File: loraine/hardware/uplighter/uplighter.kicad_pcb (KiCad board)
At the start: 2 copper layers, 50 x 50 mm, 13 parts, among them K1 CONN_3, K2 CONN_3, K3 CONN_3, U1 TL4242, U2 TL4242, U3 TL4242

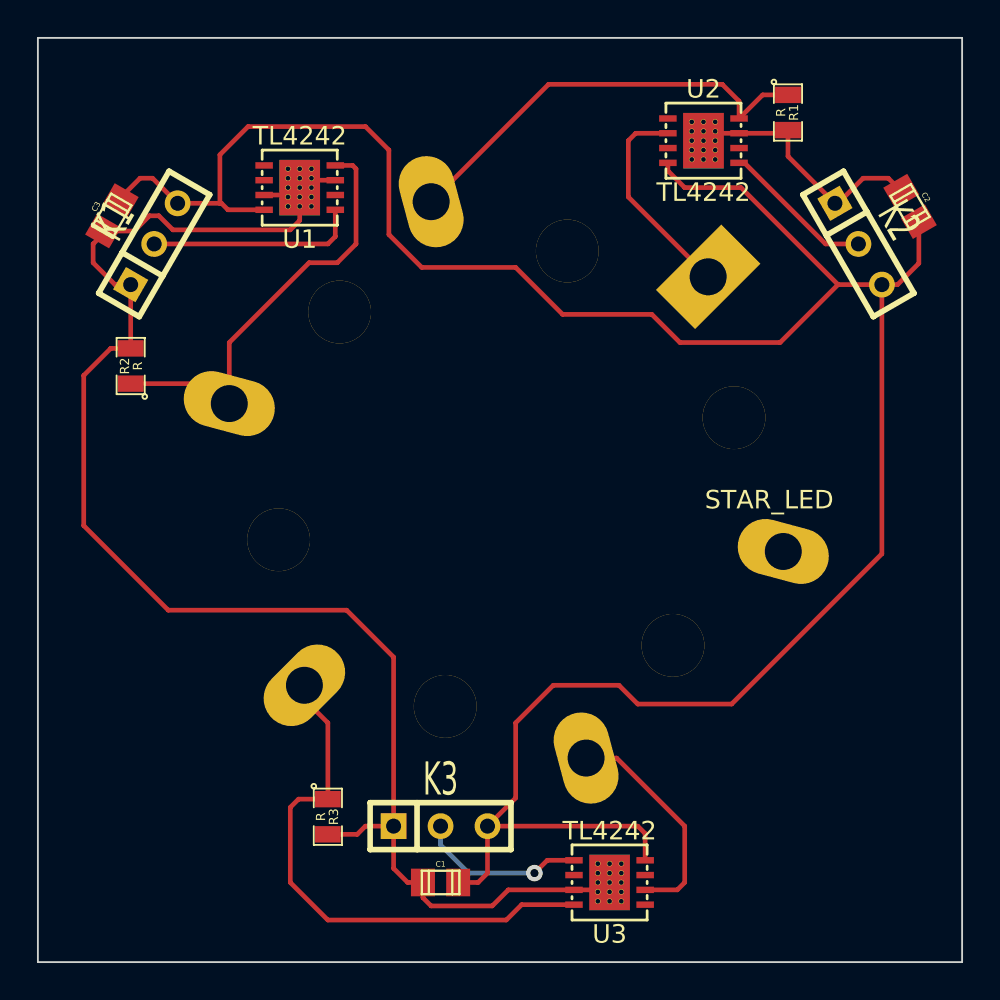
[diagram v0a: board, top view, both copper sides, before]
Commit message: Finished both PCBs apart from logos and checking
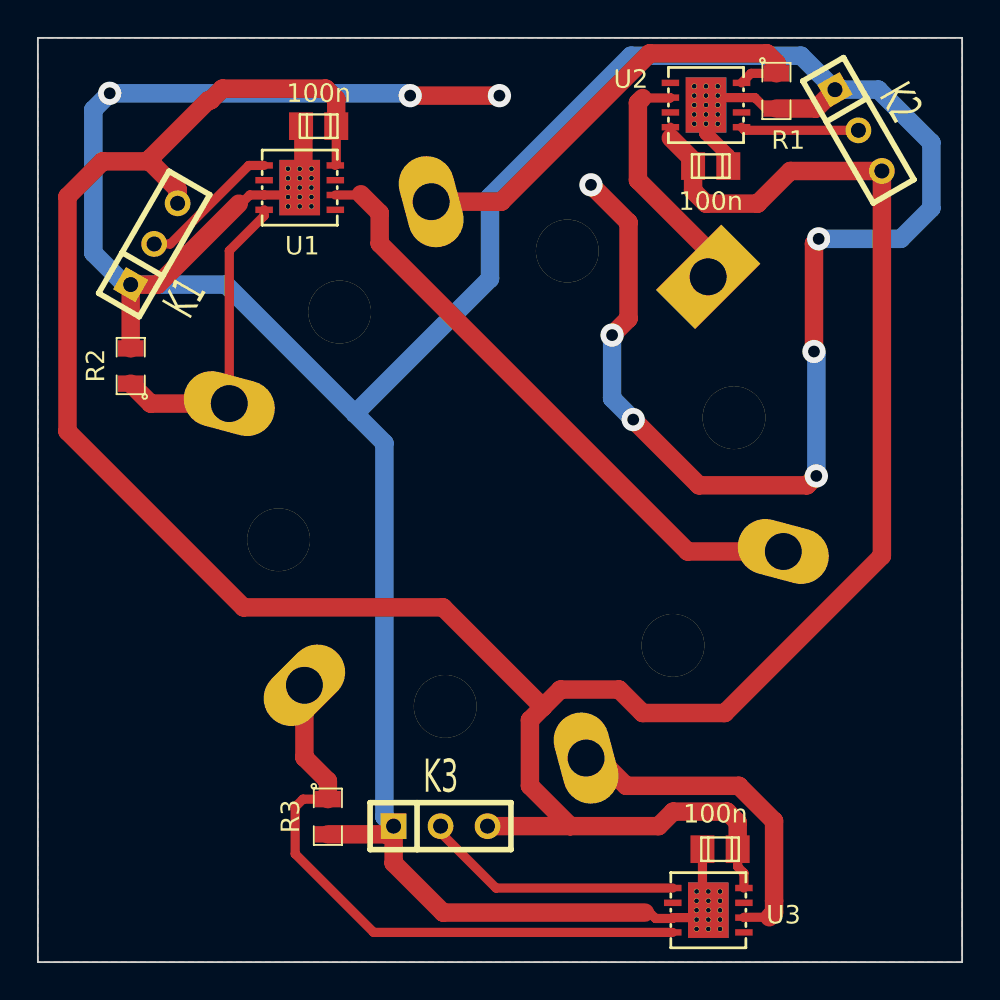
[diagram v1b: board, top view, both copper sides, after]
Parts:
- C1, C2, C3: value C -> 100n
- moved C1 15.2 mm to (136.9, 143.9)
- moved C3 12.2 mm to (115.2, 104.8), turned to 0 degrees
- moved C2 11.0 mm to (136.4, 106.9), turned to 180 degrees
- moved K2 6.15 mm to (144.4, 105.0)
- moved U3 5.55 mm to (136.3, 147.2)
- moved U2 1.93 mm to (136.1, 103.6)
- moved R1 1.32 mm to (140.0, 102.9)
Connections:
- net +5V renamed VCC
- U1 pad 2: Net-(U1-Pad2) -> (no net)
- U1 pad 5: Net-(U1-Pad5) -> (no net)
- U1 pad 7: Net-(U1-Pad7) -> (no net)
- U2 pad 2: Net-(U2-Pad2) -> (no net)
- U2 pad 5: Net-(U2-Pad5) -> (no net)
- U2 pad 7: Net-(U2-Pad7) -> (no net)
- U3 pad 2: Net-(U3-Pad2) -> (no net)
- U3 pad 5: Net-(U3-Pad5) -> (no net)
- U3 pad 7: Net-(U3-Pad7) -> (no net)
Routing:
- net GND: track 99.3 -> 221.4 mm, vias 0 -> 9
- net VCC: track 79.6 -> 153.0 mm
- net /REF_RED: track 77.7 -> 17.0 mm
- net /LED_RED: track 0.00 -> 33.3 mm
- net /LED_BLUE: track 12.2 -> 18.8 mm
- net Net-(K3-Pad2): track 9.15 -> 14.2 mm, vias 1 -> 0
- net /REF_BLUE: track 29.5 -> 33.8 mm
- net /LED_GREEN: track 11.5 -> 13.8 mm
- net Net-(K1-Pad2): track 10.2 -> 7.96 mm
- net Net-(K2-Pad2): track 8.27 -> 6.39 mm
- net Net-(U1-Pad5): track 1.45 -> 0.00 mm
- net /REF_GREEN: track 23.8 -> 24.9 mm
- added copper zone on B.Cu, net GND
- added copper zone on F.Cu, net GND
